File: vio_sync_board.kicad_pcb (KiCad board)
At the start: 2 copper layers, 53 x 64 mm, 3 parts, among them IC1 Pololu 2595, U1 Pololu D24V5F1

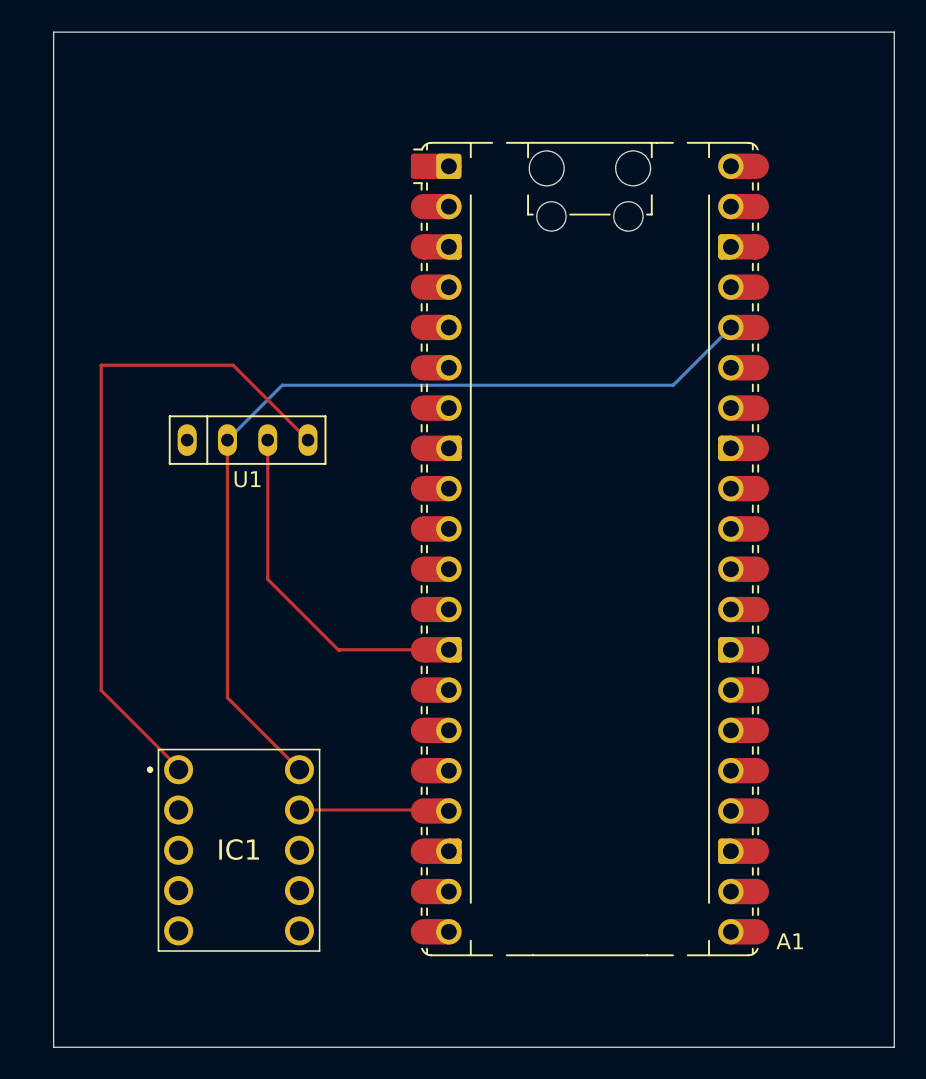
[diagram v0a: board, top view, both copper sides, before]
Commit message: layout
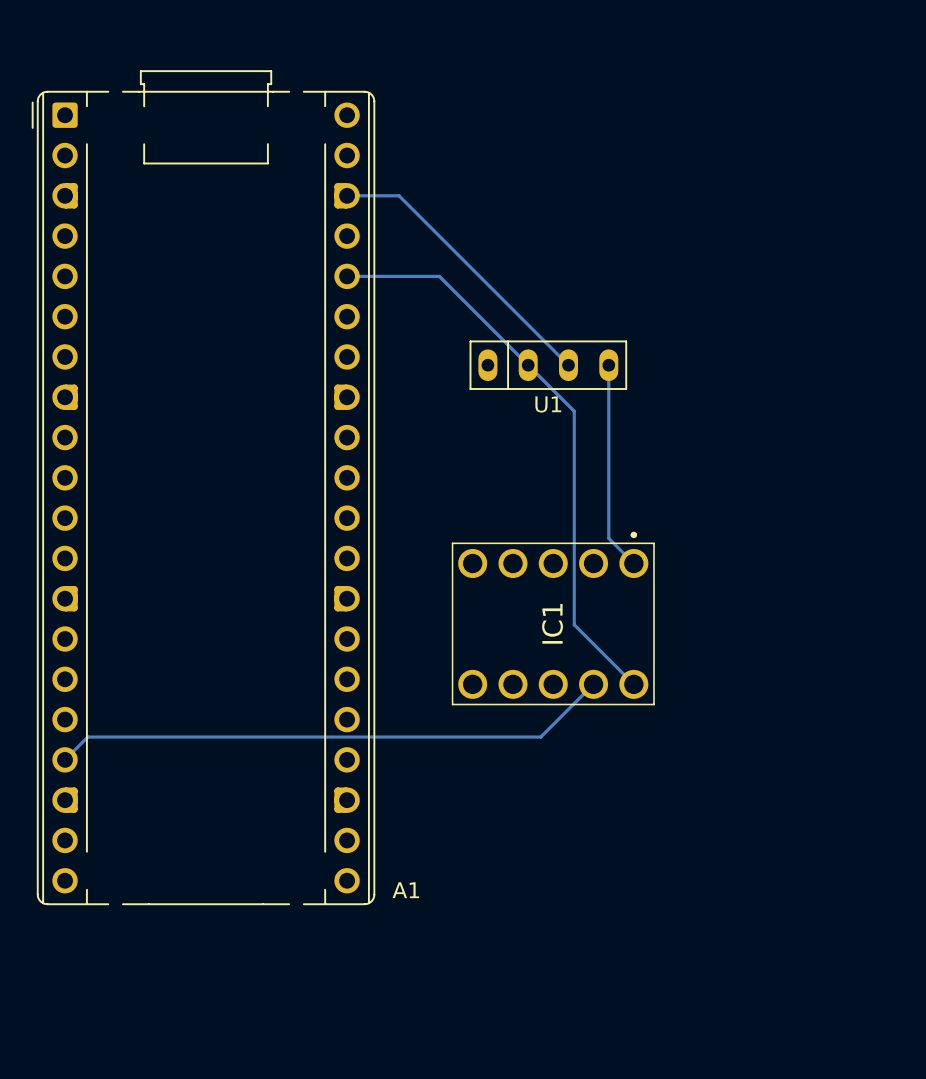
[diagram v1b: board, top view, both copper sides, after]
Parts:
- A1: footprint Module:RaspberryPi_Pico_Common_Unspecified -> Module:RaspberryPi_Pico_Common_THT
- moved A1 42.9 mm to (50.7, 50.2)
- moved IC1 31.5 mm to (86.6, 78.5), turned to -90 degrees
- moved U1 19.5 mm to (81.2, 66.0)
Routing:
- net Net-(IC1-LV): track 42.5 -> 13.2 mm
- net Net-(A1-GPIO13): track 8.64 -> 35.3 mm
- net Net-(A1-3V3): track 57.3 -> 36.6 mm
- net Net-(U1-GND): track 21.3 -> 18.4 mm
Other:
- board outline removed
